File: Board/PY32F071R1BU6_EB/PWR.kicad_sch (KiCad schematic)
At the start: 22 parts, among them J1 USB_C_Receptacle_USB2.0_16P, J3 BAT, U2 LTH7R/J, U3 XC6206P332MR-MS, U4 USBLC6-4SC6

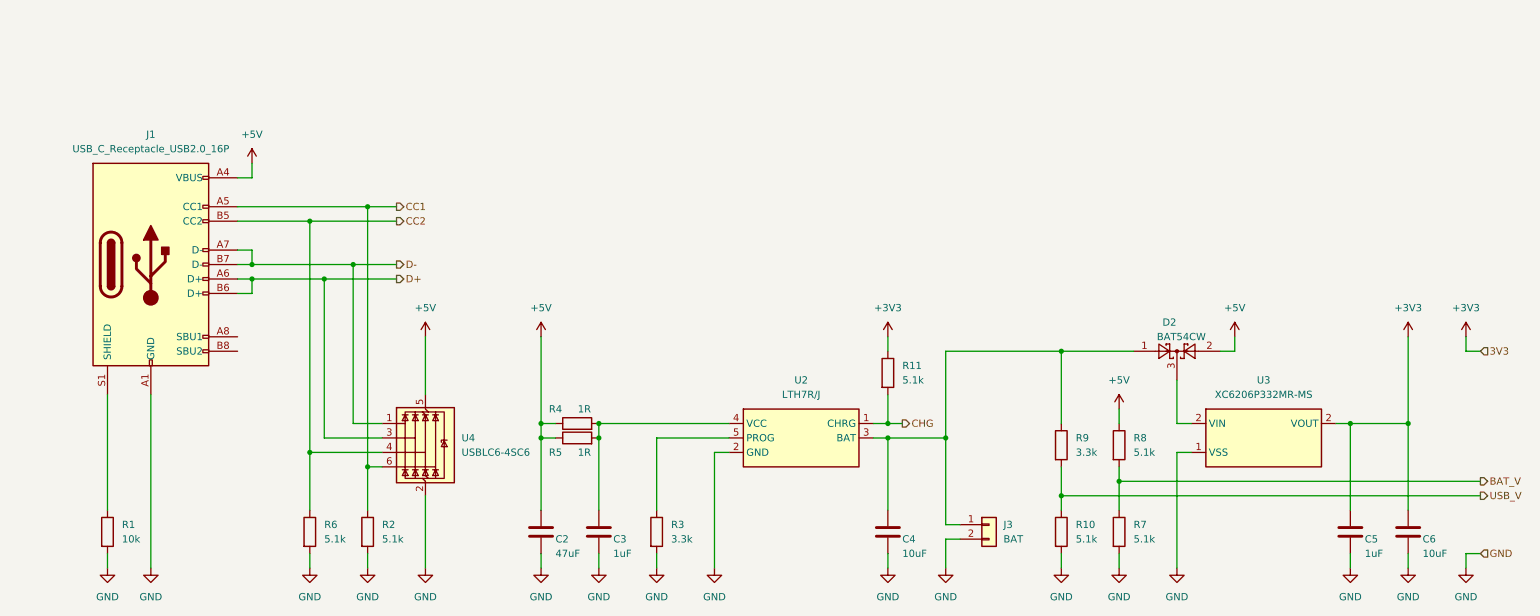
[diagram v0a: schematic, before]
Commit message: Component placement started
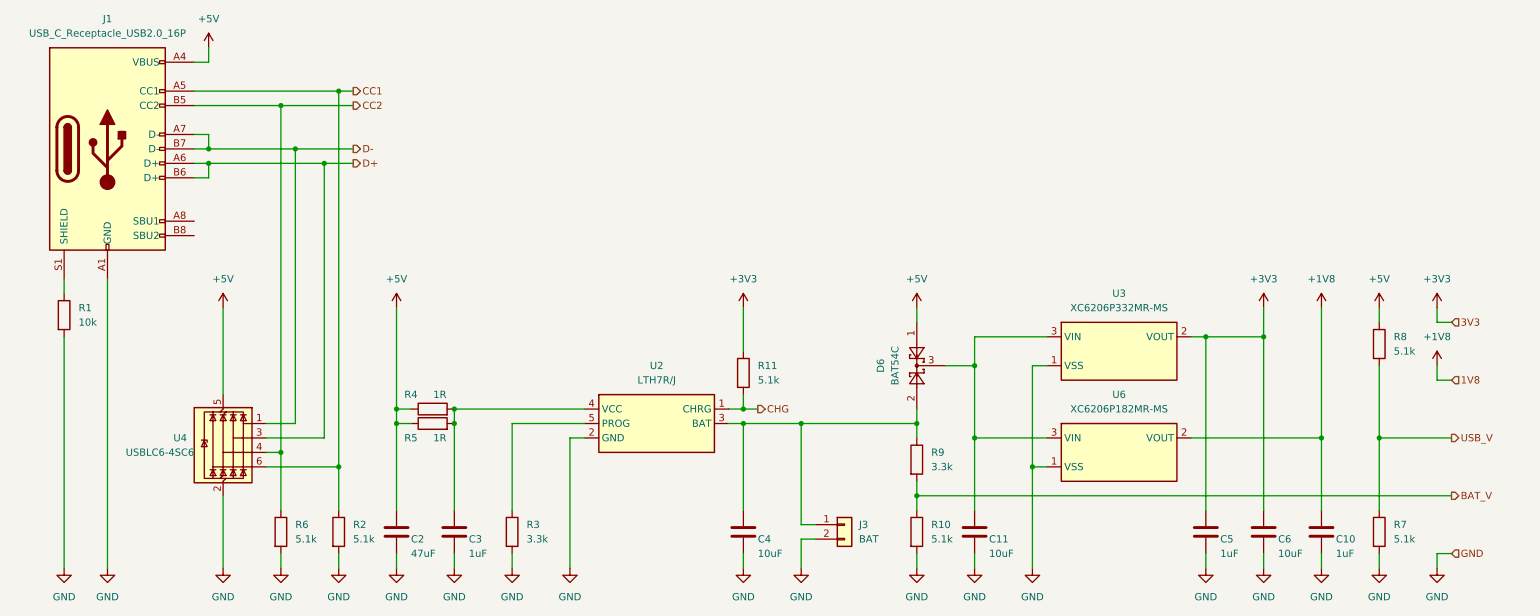
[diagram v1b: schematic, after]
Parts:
- removed D2: BAT54CW, Package_TO_SOT_SMD:SOT-323_SC-70, symbol Diode:BAT54CW
- added C10: 1uF, Capacitor_SMD:C_0603_1608Metric_Pad1.08x0.95mm_HandSolder, symbol Device:C
- added C11: 10uF, Capacitor_SMD:C_0603_1608Metric_Pad1.08x0.95mm_HandSolder, symbol Device:C
- added D6: BAT54C, Package_TO_SOT_SMD:SOT-23-3, symbol Diode:BAT54C
- added U6: XC6206P182MR-MS, Package_TO_SOT_SMD:SOT-23-3, symbol USER:XC6206P182MR-MS
- J3: footprint Connector_PinHeader_2.54mm:PinHeader_1x02_P2.54mm_Horizontal -> Connector_PinHeader_2.54mm:PinHeader_1x02_P2.54mm_Vertical
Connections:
- net +5V: now also D6.1
- net BAT_V: now also R10.1, R9.2; no longer R7.1, R8.2
- net GND: now also C10.2, C11.2, U6.1 (VSS)
- net USB_V: now also R7.1, R8.2; no longer R10.1, R9.2
- net at C4.1, J3.1 (Pin_1), R9.1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: now also D6.2
- new net: C11.1, D6.3, U3.3 (VIN), U6.3 (VIN)
- new net +1V8: C10.1, U6.2 (VOUT)
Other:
- moved on the sheet: C2, C3, C4, C5, C6, J1, J3, R1, R10, R11, R2, R3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
